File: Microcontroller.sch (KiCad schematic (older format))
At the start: 43 parts, among them CN2 CONN_RCPT_USB2.0_MINI_B_SMD_R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, M1 2N7002BK, M2 2N7002BK, Q10 2N7002BK, U2 STM32L476RGLQFP64, X1 ABM3B-16.000MHZ

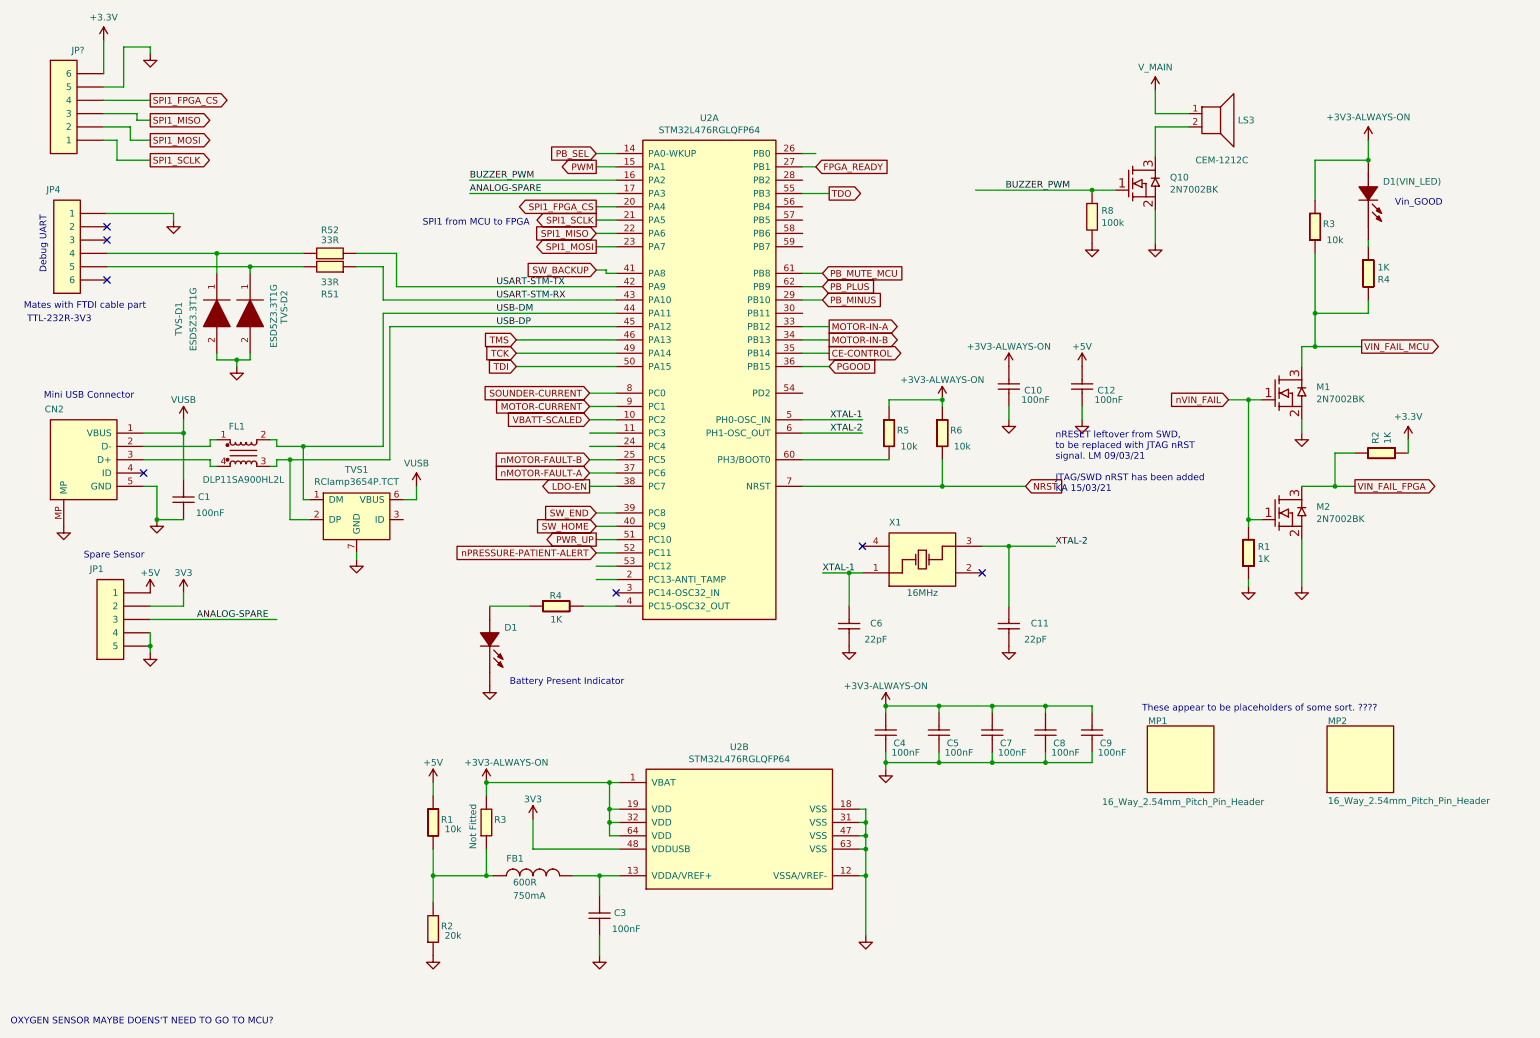
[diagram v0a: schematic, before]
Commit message: Update Microcontroller.sch
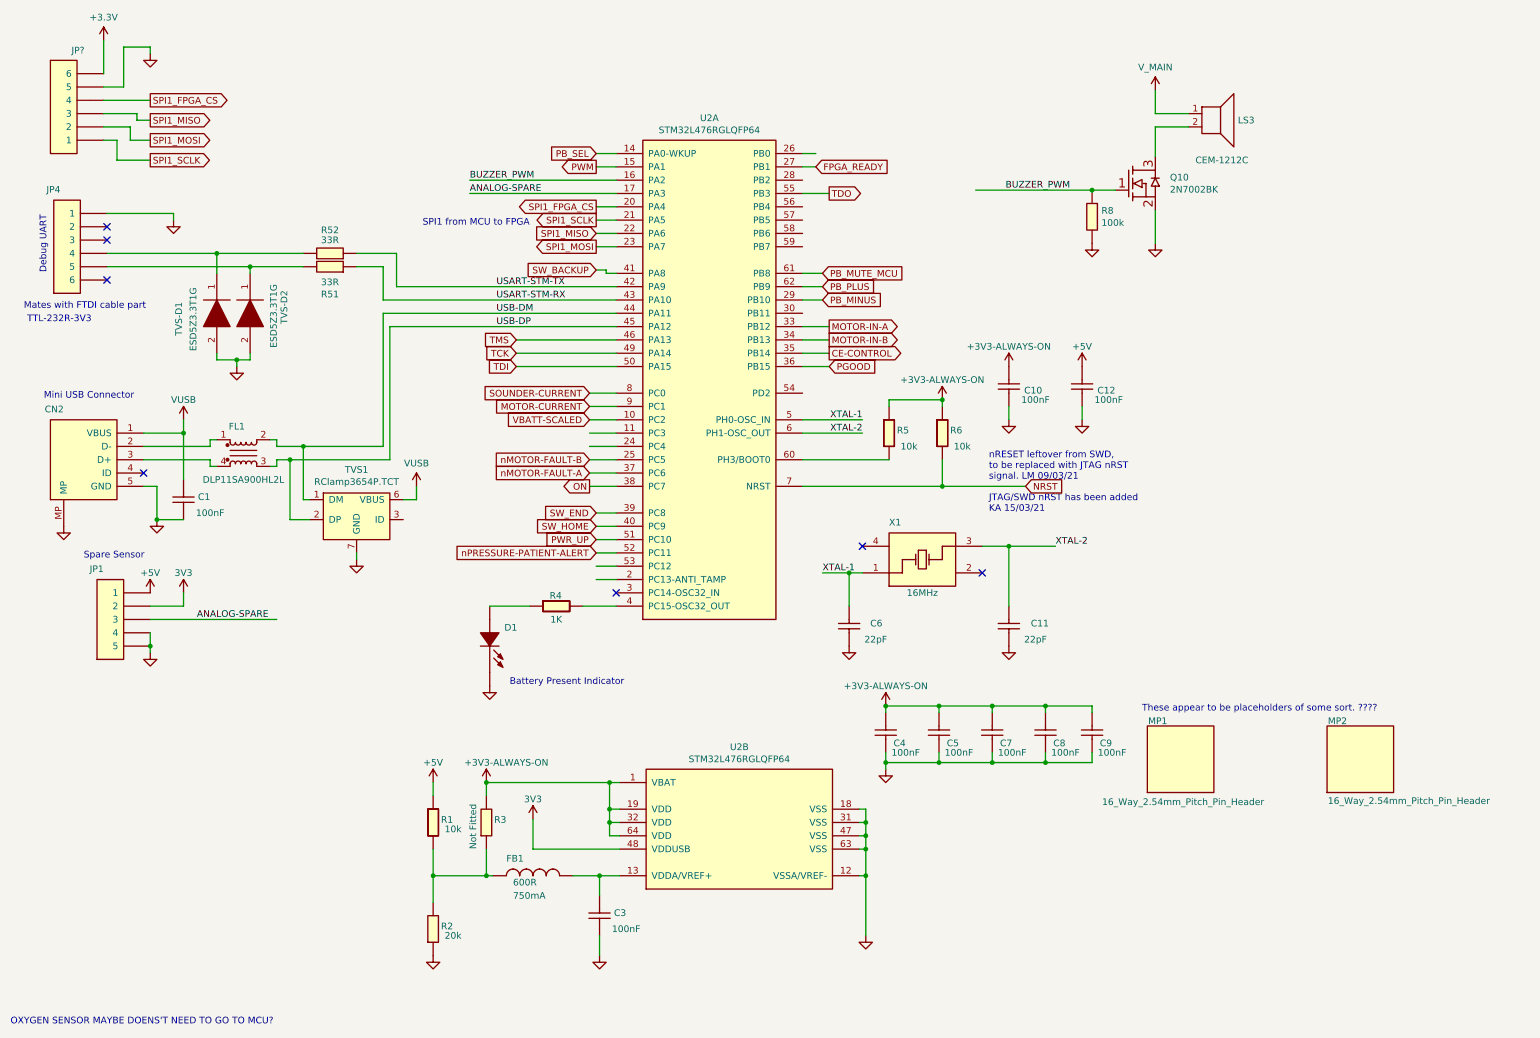
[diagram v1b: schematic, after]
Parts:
- removed D1(VIN_LED): LED_GREEN_0603_SMD, LED_SMD:LED_0603_1608Metric, symbol OpenVent:LED_GREEN_0603_SMD
- removed M1, M2: 2N7002BK, symbol OpenVent:2N7002BK
- removed R1, R2, R4: 1K_0603_Chip_Resistor,_1%,_0.1W, symbol OpenVent:1K_0603_Chip_Resistor,_1%,_0.1W
- removed R3: 10k_0603_Chip_Resistor,_1%,_0.1W, Resistor_SMD:R_0603_1608Metric, symbol OpenVent:10k_0603_Chip_Resistor,_1%,_0.1W
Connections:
- net labels added: ON
- net labels removed: LDO-EN, VIN_FAIL_FPGA, VIN_FAIL_MCU, nVIN_FAIL
- wire segments 208 -> 184
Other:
- note removed: "Vin_GOOD"
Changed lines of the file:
@@
 Text GLabel 4750 3900 0    50   Input ~ 0
 nMOTOR-FAULT-B
-Text GLabel 4750 4100 0    50   Output ~ 0
-LDO-EN
 $Comp
 L OpenVent:+5V #5V_01
@@
 	1    0    0    -1
 $EndComp
-Text GLabel 4800 4500 0    50   Output ~ 0
+Text GLabel 4800 4500 0    50   Input ~ 0
 PWR_UP
 $Comp
@@
 	4950 4000 4750 4000
 Wire Wire Line
-	4750 4100 4950 4100
-Wire Wire Line
 	4800 2100 4950 2100
 Wire Wire Line
@@
 Text GLabel 4800 1600 0    50   Input ~ 0
 PB_SEL
-$Comp
-L OpenVent:2N7002BK M2
-U 1 1 603E15FB
-P 10100 4100
-F 0 "M2" H 9990 3946 50  0000 R CNN
-F 1 "2N7002BK" H 9990 3855 50  0000 R CNN
-F 2 "" H 10100 4100 50  0000 C CNN
-F 3 "" H 10100 4100 50  0000 C CNN
-	1    10100 4100
-	-1   0    0    -1
-$EndComp
-$Comp
-L OpenVent:2N7002BK M1
-U 1 1 603F9909
-P 10100 3200
-F 0 "M1" H 9990 3046 50  0000 R CNN
-F 1 "2N7002BK" H 9990 2955 50  0000 R CNN
-F 2 "" H 10100 3200 50  0000 C CNN
-F 3 "" H 10100 3200 50  0000 C CNN
-	1    10100 3200
-	-1   0    0    -1
-$EndComp
-$Comp
-L OpenVent:1K_0603_Chip_Resistor,_1%,_0.1W R4
-U 1 1 6042A601
-P 10700 2600
-AR Path="/5F988182/6042A601" Ref="R4"  Part="1"
-AR Path="/5F99D63D/6042A601" Ref="R?"  Part="1"
-F 0 "R4" V 10754 2570 50  0000 L CNN
-F 1 "1K_0603_Chip_Resistor,_1%,_0.1W" H 10700 2600 50  0001 C CNN
-F 2 "" H 10700 2600 60  0001 C CNN
-F 3 "" H 10700 2600 60  0001 C CNN
-F 4 "1K" V 10845 2570 50  0000 L CNN "Val"
-F 5 "1%" H 10700 2600 50  0001 C CNN "Tolerance"
-F 6 "0.1W" H 10700 2600 50  0001 C CNN "Watt"
-	1    10700 2600
-	0    1    -1   0
-$EndComp
-$Comp
-L OpenVent:1K_0603_Chip_Resistor,_1%,_0.1W R2
-U 1 1 60436A21
-P 10600 3750
-AR Path="/5F988182/60436A21" Ref="R2"  Part="1"
-AR Path="/5F99D63D/60436A21" Ref="R?"  Part="1"
-F 0 "R2" V 10654 3720 50  0000 L CNN
-F 1 "1K_0603_Chip_Resistor,_1%,_0.1W" H 10600 3750 50  0001 C CNN
-F 2 "" H 10600 3750 60  0001 C CNN
-F 3 "" H 10600 3750 60  0001 C CNN
-F 4 "1K" V 10745 3720 50  0000 L CNN "Val"
-F 5 "1%" H 10600 3750 50  0001 C CNN "Tolerance"
-F 6 "0.1W" H 10600 3750 50  0001 C CNN "Watt"
-	1    10600 3750
-	1    0    0    -1
-$EndComp
-$Comp
-L OpenVent:10k_0603_Chip_Resistor,_1%,_0.1W R3
-U 1 1 604A9F02
-P 10100 2250
-F 0 "R3" V 10250 2000 50  0000 L BNN
-F 1 "10k_0603_Chip_Resistor,_1%,_0.1W" V 10100 2100 50  0001 C CNN
-F 2 "Resistor_SMD:R_0603_1608Metric" H 10000 2110 50  0001 C CNN
-F 3 "" H 10000 2110 50  0001 C CNN
-F 4 "1%" V 4500 -2750 50  0001 C CNN "Tolerance"
-F 5 "10k" V 10100 2000 50  0000 C CNN "Val"
-F 6 "0.1W" H 10100 2250 50  0001 C CNN "Watt"
-	1    10100 2250
-	0    -1   -1   0
-$EndComp
-Text GLabel 9550 3450 0    50   Input ~ 0
-nVIN_FAIL
-Text GLabel 10550 3050 2    50   Output ~ 0
-VIN_FAIL_MCU
-$Comp
-L OpenVent:GND #GND_?
-U 1 1 606DD025
-P 10100 4850
-F 0 "#GND_?" H 10100 4600 50  0001 C CNN
-F 1 "GND" H 10100 4700 50  0001 C CNN
-F 2 "" H 10100 4850 50  0000 C CNN
-F 3 "" H 10100 4850 50  0000 C CNN
-	1    10100 4850
-	1    0    0    -1
-$EndComp
-$Comp
-L OpenVent:GND #GND_?
-U 1 1 6071B931
-P 10100 3700
-F 0 "#GND_?" H 10100 3450 50  0001 C CNN
-F 1 "GND" H 10100 3550 50  0001 C CNN
-F 2 "" H 10100 3700 50  0000 C CNN
-F 3 "" H 10100 3700 50  0000 C CNN
-	1    10100 3700
-	1    0    0    -1
-$EndComp
-Wire Wire Line
-	10100 3600 10100 3700
-Wire Wire Line
-	10600 2700 10600 2800
-Wire Wire Line
-	10100 3050 10100 3200
-Wire Wire Line
-	10600 2300 10600 2250
-$Comp
-L OpenVent:+3V3-ALWAYS-ON #PWR?
-U 1 1 60842A63
-P 10600 1500
-F 0 "#PWR?" H 10600 1400 50  0001 C CNN
-F 1 "+3V3-ALWAYS-ON" H 10600 1673 50  0000 C CNN
-F 2 "" H 10600 1500 50  0001 C CNN
-F 3 "" H 10600 1500 50  0001 C CNN
-	1    10600 1500
-	1    0    0    -1
-$EndComp
-$Comp
-L OpenVent:+3.3V #PWR?
-U 1 1 608506F9
-P 10900 3750
-F 0 "#PWR?" H 10900 3600 50  0001 C CNN
-F 1 "+3.3V" H 10900 3923 50  0000 C CNN
-F 2 "" H 10900 3750 50  0001 C CNN
-F 3 "" H 10900 3750 50  0001 C CNN
-	1    10900 3750
-	1    0    0    -1
-$EndComp
-Wire Wire Line
-	10900 3850 10900 3750
-Text GLabel 10500 4100 2    50   Output ~ 0
-VIN_FAIL_FPGA
-Wire Wire Line
-	10500 3850 10350 3850
-Wire Wire Line
-	10350 3850 10350 4100
-Wire Wire Line
-	10350 4100 10500 4100
-Wire Wire Line
-	9700 4350 9800 4350
-$Comp
-L OpenVent:GND #GND_?
-U 1 1 6071A6F8
-P 9700 4850
-F 0 "#GND_?" H 9700 4600 50  0001 C CNN
-F 1 "GND" H 9700 4700 50  0001 C CNN
-F 2 "" H 9700 4850 50  0000 C CNN
-F 3 "" H 9700 4850 50  0000 C CNN
-	1    9700 4850
-	1    0    0    -1
-$EndComp
-$Comp
-L OpenVent:1K_0603_Chip_Resistor,_1%,_0.1W R1
-U 1 1 6045AB44
-P 9800 4500
-AR Path="/5F988182/6045AB44" Ref="R1"  Part="1"
-AR Path="/5F99D63D/6045AB44" Ref="R?"  Part="1"
-F 0 "R1" V 9854 4470 50  0000 L CNN
-F 1 "1K_0603_Chip_Resistor,_1%,_0.1W" H 9800 4500 50  0001 C CNN
-F 2 "" H 9800 4500 60  0001 C CNN
-F 3 "" H 9800 4500 60  0001 C CNN
-F 4 "1K" V 9945 4470 50  0000 L CNN "Val"
-F 5 "1%" H 9800 4500 50  0001 C CNN "Tolerance"
-F 6 "0.1W" H 9800 4500 50  0001 C CNN "Watt"
-	1    9800 4500
-	0    1    1    0
-$EndComp
-Wire Wire Line
-	9550 3450 9700 3450
-Wire Wire Line
-	10100 4100 10350 4100
-Connection ~ 10350 4100
-Wire Wire Line
-	9700 4350 9700 3450
-Connection ~ 9700 3450
-Wire Wire Line
-	9700 3450 9800 3450
-Wire Wire Line
-	10100 4500 10100 4850
-Wire Wire Line
-	10200 2350 10200 2800
-Wire Wire Line
-	10600 2800 10200 2800
-Wire Wire Line
-	10200 1950 10200 1650
-Wire Wire Line
-	10200 1650 10600 1650
-Wire Wire Line
-	10600 1500 10600 1650
-Text Notes 10800 2000 0    50   ~ 0
-Vin_GOOD
-Wire Wire Line
-	9700 4850 9700 4800
-Wire Wire Line
-	9700 4400 9700 4350
-Connection ~ 9700 4350
-Wire Wire Line
-	10100 3050 10200 3050
-Wire Wire Line
-	10200 2800 10200 3050
-Connection ~ 10200 2800
-Connection ~ 10200 3050
-Wire Wire Line
-	10200 3050 10550 3050
-Connection ~ 10600 1650
-$Comp
-L OpenVent:LED_GREEN_0603_SMD D?
-U 1 1 604063DB
-P 10600 1650
-AR Path="/604063DB" Ref="D?"  Part="1"
-AR Path="/5F988182/604063DB" Ref="D1(VIN_LED)"  Part="1"
-F 0 "D1(VIN_LED)" V 10790 1760 50  0000 L BNN
-F 1 "LED_GREEN_0603_SMD" V 10890 1760 60  0001 C CNN
-F 2 "LED_SMD:LED_0603_1608Metric" H 10890 1760 50  0001 C CNN
-F 3 "https://www.rohm.com/datasheet/SML-D12M8W(C)/sml-d12x8(c)-e" H 10890 1760 50  0001 C CNN
-F 4 "" V 10900 1900 50  0000 C CNN "Val"
-F 5 "GREEN" H 10600 1650 50  0001 C CNN "Colour"
-F 6 "SML-D12M8WT86C" H 10600 1650 50  0001 C CNN "Mfr_PN"
-F 7 "LED YELLOW/GREEN 1608 SMD" H 10600 1650 50  0001 C CNN "Desc"
-F 8 "Yellow-Green 572nm LED Indication - Discrete 2.2V 0603 (1608 Metric)" H 10600 1650 50  0001 C CNN "Detailed"
-F 9 "DigiKey" H 10600 1650 50  0001 C CNN "DistName"
-F 10 "SML-D12M8WT86CTR-ND" H 10600 1650 50  0001 C CNN "Dist_PN"
-F 11 "Rohm Semiconductor" H 10600 1650 50  0001 C CNN "Mfr"
-	1    10600 1650
-	0    1    1    0
-$EndComp
-Text Notes 8250 4150 0    50   ~ 0
+Text Notes 7750 4300 0    50   ~ 0
 nRESET leftover from SWD,\nto be replaced with JTAG nRST\nsignal. LM 09/03/21\n\nJTAG/SWD nRST has been added \nKA 15/03/21\n
 Text GLabel 6450 1700 2    50   Input ~ 0
@@
 Wire Wire Line
 	2200 2450 2600 2450
+Wire Wire Line
+	4750 4100 4950 4100
+Text GLabel 4750 4100 0    50   Output ~ 0
+ON
 $EndSCHEMATC
